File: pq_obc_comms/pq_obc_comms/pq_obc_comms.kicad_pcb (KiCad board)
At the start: 4 copper layers, 40 x 40 mm, 66 parts, among them J1 Conn_01x10, J2 Conn_01x10, J3 Conn_01x10, J4 Conn_01x10, J6 U.FL-R-SMT-1_10, U1 STM32L476RGTx, U2 SX1262IMLTRT, U3 BD2232G-GTR, U4 BD2232G-GTR, U5 BGS12PL6E6327XTSA1, U7 BD2232G-GTR, X1 ECS-120-18-33-JEM-TR3, X2 FA-128_32.0000MF20X-K5, X3 ABS09-32.768KHZ-7-T

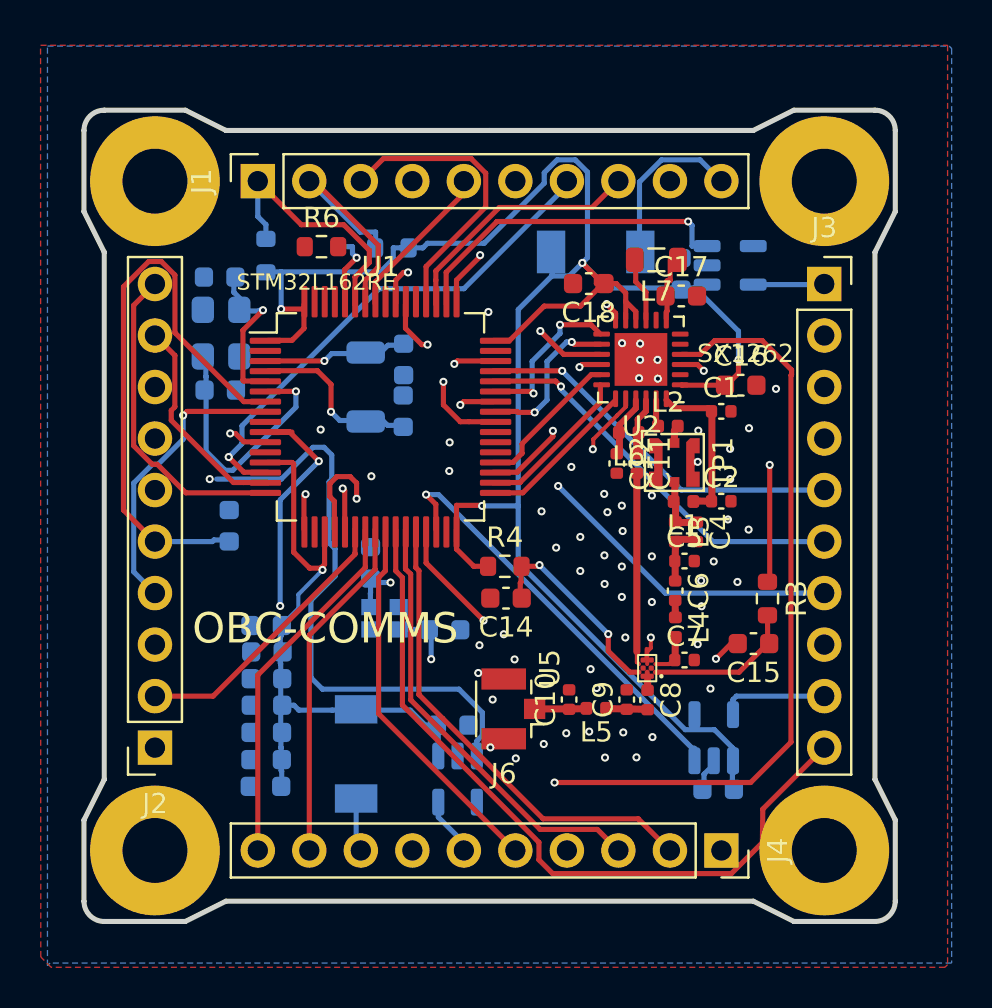
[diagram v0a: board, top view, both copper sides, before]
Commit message: OBC board revision 3 finished
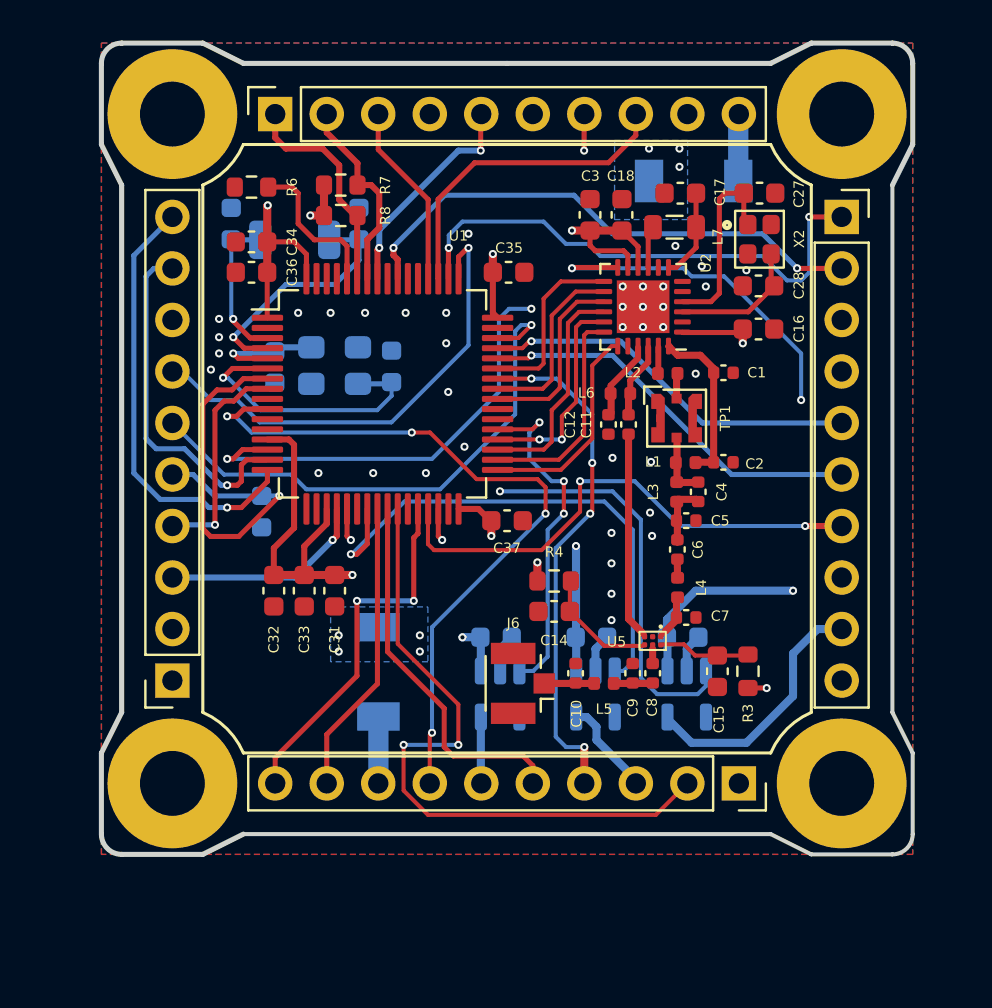
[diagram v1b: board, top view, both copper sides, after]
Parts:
- added C3: 100nF, Capacitor_SMD:C_0603_1608Metric, F.Cu at (104.1, 48.5)
- C27, C28, C31, C32, C33, C34, C35, C36, C37, R7, R8: moved to F.Cu
- X2: footprint easyeda:FA128320000MF20XK5 -> GGS_Miscellaneous:EPSON_FA128
- moved C27 26.5 mm to (112.4, 47.4)
- moved X2 26.3 mm to (112.4, 49.7), turned to -90 degrees
- moved C35 25.6 mm to (100.1, 51.3), turned to 0 degrees
- moved C36 24.0 mm to (87.4, 51.3)
- moved C28 23.5 mm to (112.4, 52.0), turned to 180 degrees
- moved C34 22.9 mm to (87.4, 49.8)
- moved U4 22.2 mm to (104.4, 72.1), turned to -90 degrees
- moved C44 18.5 mm to (104.2, 69.3), turned to 0 degrees
- moved C37 17.7 mm to (100.0, 63.5), turned to 0 degrees
- moved C38 10.8 mm to (86.4, 48.9), turned to 90 degrees
- moved C39 9.50 mm to (92.7, 48.9)
- moved C41 8.53 mm to (94.3, 55.9), turned to 90 degrees
- moved X3 8.06 mm to (89.5, 49.7), turned to 0 degrees
- moved C43 7.71 mm to (108.7, 69.3)
- moved D1 5.96 mm to (109.2, 46.8)
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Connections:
- net Net-(R3-Pad1) renamed /DIO2
- net Net-(U5-Pad4) renamed /RFswitch_Vcc
- D1 pad 1: 3V3 -> 3V3_PERM
- J3 pad 10: unconnected-(J3-Pad10) -> GND
- J4 pad 2: STM32_PD2 -> STM32_PB0
- U1 pad 10: SEL_PH3 -> SEL_PH0
- U1 pad 11: /PoL_P/L_EN -> unconnected-(U1-Pad11)
- U1 pad 22: MPPT_X -> unconnected-(U1-Pad22)
- U1 pad 23: MPPT_Z -> /PoL_ADCS_POWER_EN
- U1 pad 26: EPS_RST -> STM32_PB0
- U1 pad 27: MPPT_Y -> unconnected-(U1-Pad27)
- U1 pad 37: unconnected-(U1-Pad37) -> /PoL_P/L_EN
- U1 pad 41: /BUSY -> /SX1262_BUSY
- U1 pad 54: STM32_PD2 -> unconnected-(U1-Pad54)
- U1 pad 8: CHGOFF -> CHRGOFF
- U4 pad 3: P/L2BURN_OBC -> /PoL_ADCS_POWER_EN
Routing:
- net VCC: track 138.6 -> 63.3 mm, vias 5 -> 18
- net STM32_PD2: track 49.0 -> 0.00 mm, vias 1 -> 0
- net /XTB: track 48.8 -> 9.60 mm, vias 2 -> 0
- net SOLAR_Z: track 37.1 -> 0.00 mm
- net unconnected-(U1-Pad17): track 33.5 -> 0.00 mm, vias 2 -> 0
- net STM32_PB0: track 0.00 -> 32.9 mm, vias 0 -> 2
- net STM32_PA15: track 0.00 -> 25.9 mm, vias 0 -> 2
- net /PoL_ADCS_POWER_EN: track 0.00 -> 25.9 mm, vias 0 -> 1
- net ADCS_POWER: track 25.3 -> 4.79 mm
- net /PoL_P/L_EN: track 34.2 -> 17.0 mm, vias 2 -> 3
- net /XTA: track 23.5 -> 6.70 mm, vias 2 -> 0
- net P/L2BURN_OBC: track 16.5 -> 0.00 mm, vias 1 -> 0
- net CHGOFF: track 14.6 -> 0.00 mm, vias 1 -> 0
- net /DIO2: track 19.4 -> 33.4 mm, vias 2 -> 3
- net MPPT_X: track 14.0 -> 0.00 mm
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- added copper zone on B.Cu, net VCC
- added copper zone on In2.Cu, net VCC
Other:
- board text removed: "12MHz"
- board text removed: "32.7KHz"
- board text removed: "32MHz"
- board text removed: "BD2232G"
- board text removed: "BurnCOMMS"
- board text removed: "D-VCC"
- board text removed: "D-VCCTest"
- board text removed: "OBC-COMMS"
- board text removed: "PL2BURN"
- board text removed: "PL2VCC"
- board text removed: "STM32L162RE"
- board text removed: "SX1262"
